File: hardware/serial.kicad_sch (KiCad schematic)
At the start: 20 parts, among them J2 USB_B, J3 Conn_01x04, U29 W65C51NxP, U30 MCP2221AxP, X2 1.8432MHz

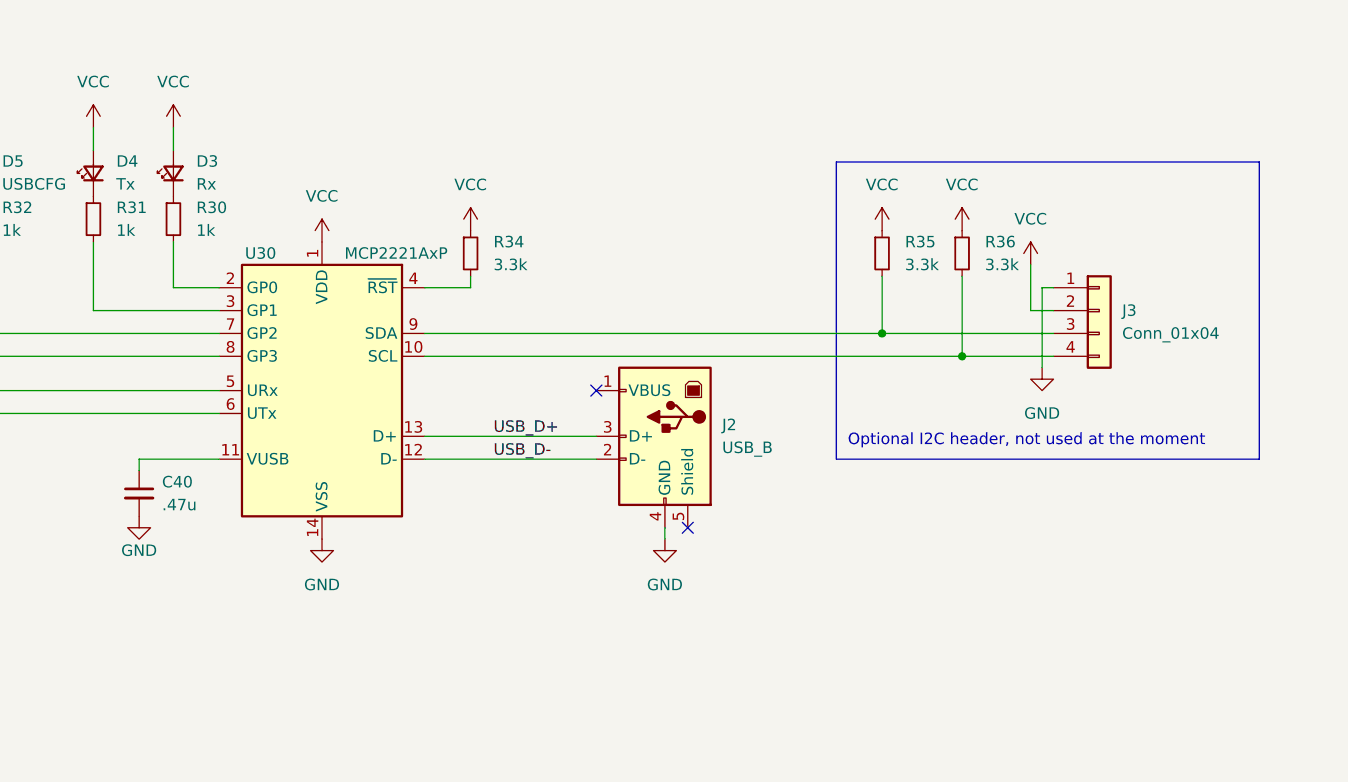
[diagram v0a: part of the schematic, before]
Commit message: Episode 30
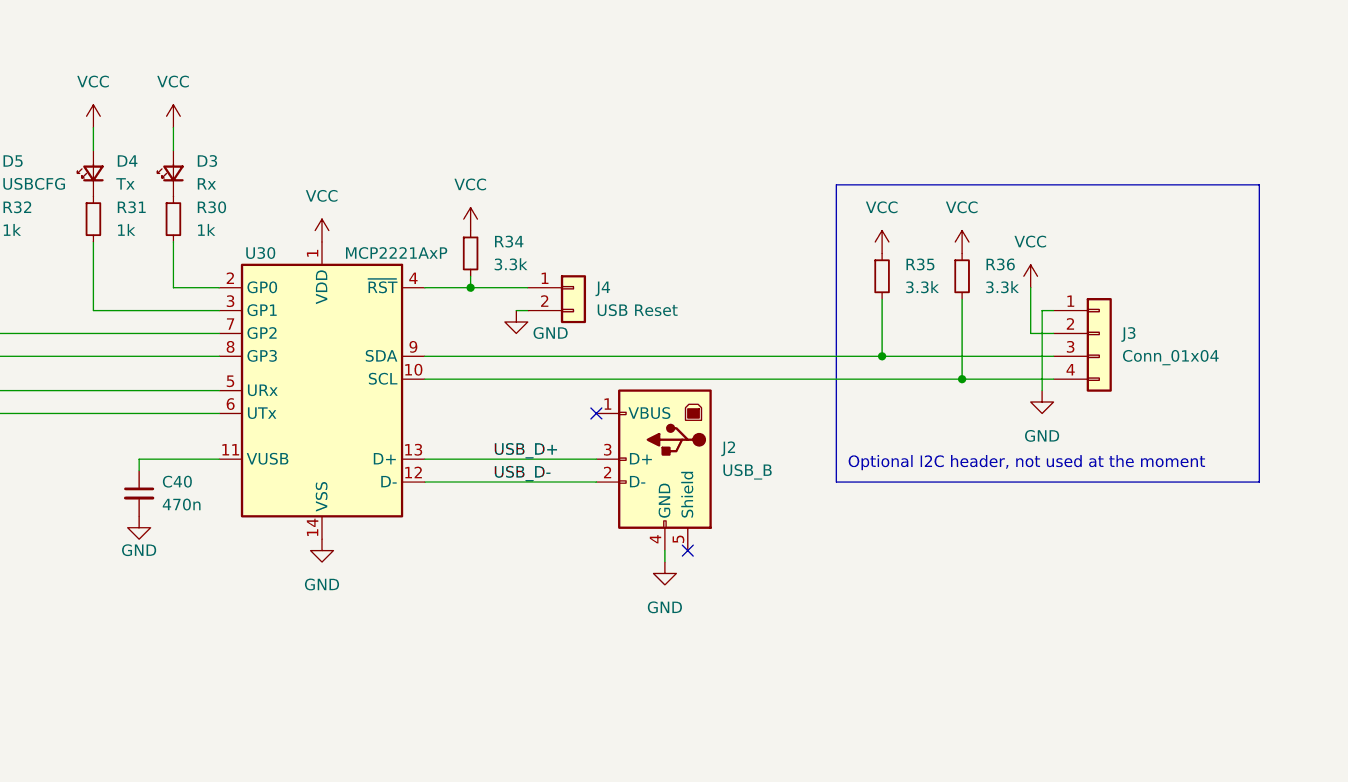
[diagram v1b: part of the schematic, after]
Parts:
- added J4: USB Reset, symbol Connector_Generic:Conn_01x02
- C40: value .47u -> 470n
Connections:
- net GND: now also J4.2 (Pin_2)
- net at R34.2, U30.4 (~{RST}): now also J4.1 (Pin_1)
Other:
- moved on the sheet: J2, J3, R35, R36
